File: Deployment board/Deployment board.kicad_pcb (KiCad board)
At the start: 2 copper layers, 43 x 51.5 mm, 28 parts, among them J1 Conn_01x04, J2 Conn_01x04, J3 Conn_01x02, J4 Conn_01x02, J5 Conn_01x02, J6 REMOVE BEFORE FLIGHT, M1 Motor_Servo, Q1 IRLR7843, Q2 IRLR7843, Q3 To be determined

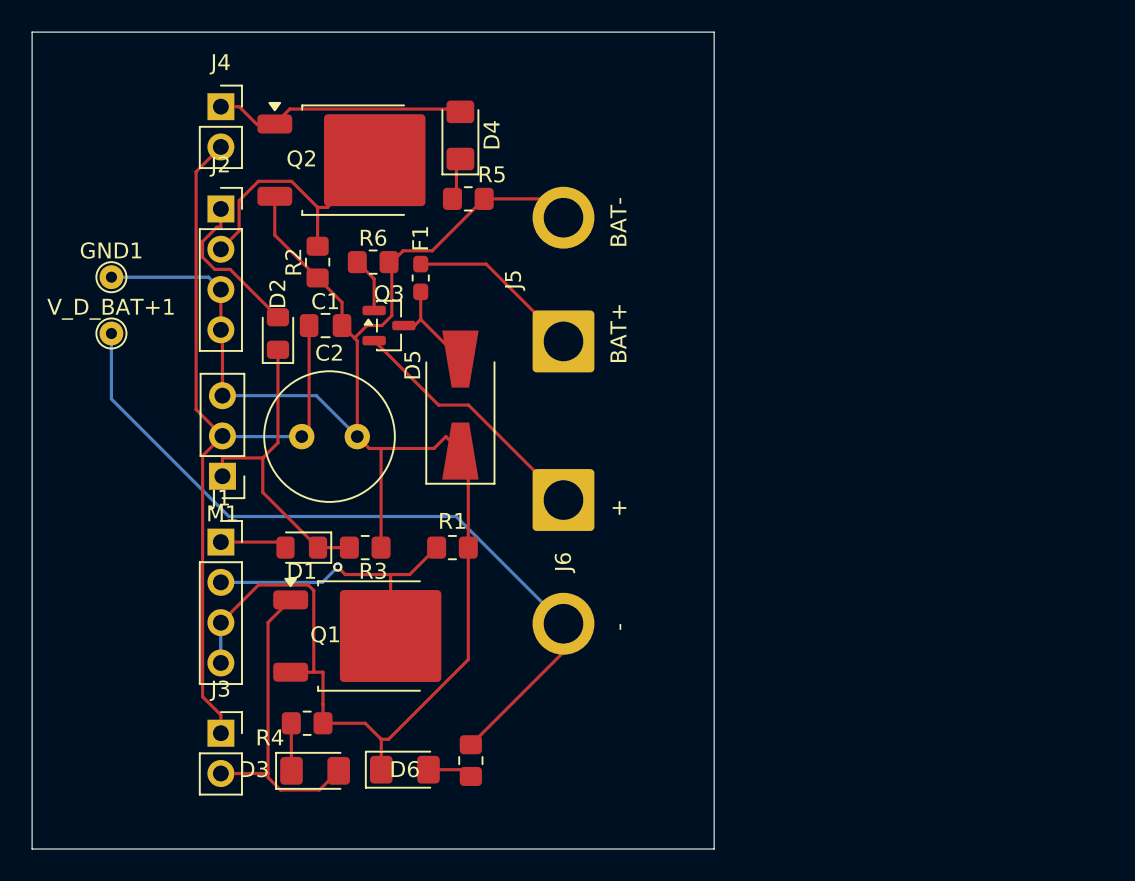
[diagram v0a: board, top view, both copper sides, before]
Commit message: jpush
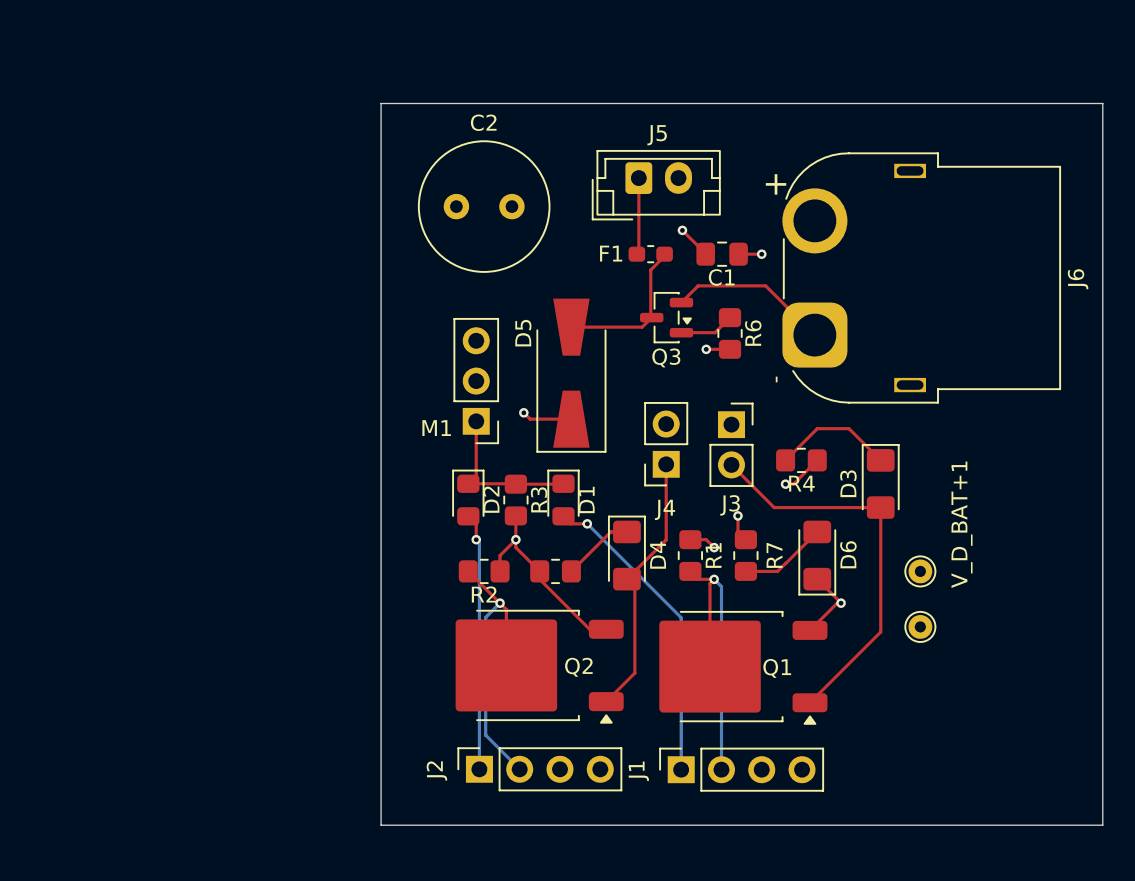
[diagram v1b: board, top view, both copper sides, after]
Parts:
- J5: footprint Connector_Wire:SolderWire-2sqmm_1x02_P7.8mm_D2mm_OD3.9mm -> Connector_JST:JST_EH_B2B-EH-A_1x02_P2.50mm_Vertical
- J6: footprint Connector_Wire:SolderWire-2sqmm_1x02_P7.8mm_D2mm_OD3.9mm -> Connector_AMASS:AMASS_XT60PW-F_1x02_P7.20mm_Horizontal
- moved GND1 55.6 mm to (71.5, 141.0), turned to 90 degrees
- moved V_D_BAT+1 53.2 mm to (71.5, 137.5)
- moved D3 40.0 mm to (69.0, 132.0), turned to -90 degrees
- moved J2 38.9 mm to (43.7, 150.0), turned to 90 degrees
- moved J3 37.6 mm to (59.6, 128.2)
- moved J4 36.0 mm to (55.5, 130.8), turned to 180 degrees
- moved R4 35.3 mm to (64.0, 130.5)
- moved Q2 33.6 mm to (46.7, 143.4), turned to 180 degrees
- moved J1 32.4 mm to (56.4, 150.0), turned to 90 degrees
- moved D6 29.3 mm to (65.0, 136.5), turned to 90 degrees
- moved D4 28.5 mm to (53.0, 136.5), turned to -90 degrees
- moved C1 25.4 mm to (59.0, 117.5), turned to 180 degrees
- moved R5 24.1 mm to (48.5, 137.5), turned to 180 degrees
- moved R6 22.9 mm to (59.5, 122.5), turned to -90 degrees
- moved Q1 22.7 mm to (59.5, 143.5), turned to 180 degrees
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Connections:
- C1 pad 1: V_Ｄ_BAT+ -> V_D_BAT+
- C2 pad 1: V_Ｄ_BAT+ -> V_D_BAT+
- J3 pad 1: V_Ｄ_BAT+ -> V_D_BAT+
- J4 pad 2: V_Ｄ_BAT+ -> V_D_BAT+
- M1 pad 2: V_Ｄ_BAT+ -> V_D_BAT+
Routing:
- net V_Ｄ_BAT+: track 51.5 -> 0.00 mm
- net V_D_BAT+: track 48.5 -> 70.4 mm, vias 0 -> 2
- net GND: track 120.9 -> 139.2 mm, vias 0 -> 7
- net Main_AV_PWM_Servo: track 4.22 -> 19.6 mm, vias 0 -> 1
- net Net-(D1-K): track 20.0 -> 10.2 mm
- net Backup_AV_PWM_Servo: track 9.99 -> 16.2 mm, vias 0 -> 1
- net Net-(J5-Pin_1): track 11.0 -> 4.85 mm
- net Net-(J6-A): track 16.1 -> 10.1 mm
- net Net-(D3-K): track 3.01 -> 7.66 mm
- net Net-(D3-A): track 20.0 -> 24.7 mm
- net Net-(D5-A2): track 6.50 -> 9.70 mm
- net Net-(D6-A): track 2.85 -> 5.53 mm
- net Backup_AV_FIRE: track 17.0 -> 18.7 mm, vias 0 -> 1
- net Net-(D4-K): track 3.07 -> 4.53 mm
- net Net-(D4-A): track 16.0 -> 16.9 mm
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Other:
- board size 43 x 51.5 mm -> 45.5 x 45.5 mm
- copper layers 2 -> 4
- board text removed: "+"
- board text removed: "-"
- board text removed: "BAT+"
- board text removed: "BAT-"

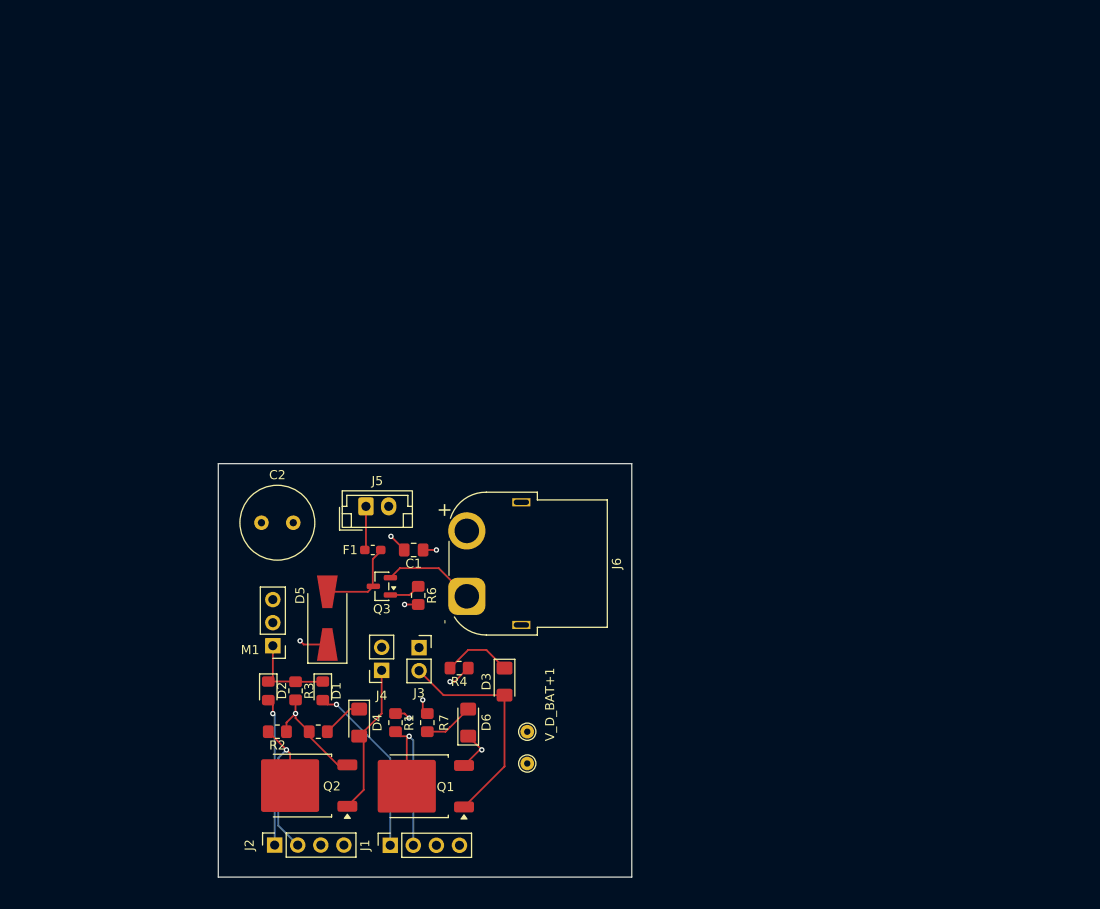
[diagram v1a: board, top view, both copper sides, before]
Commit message: finish deployment pcb
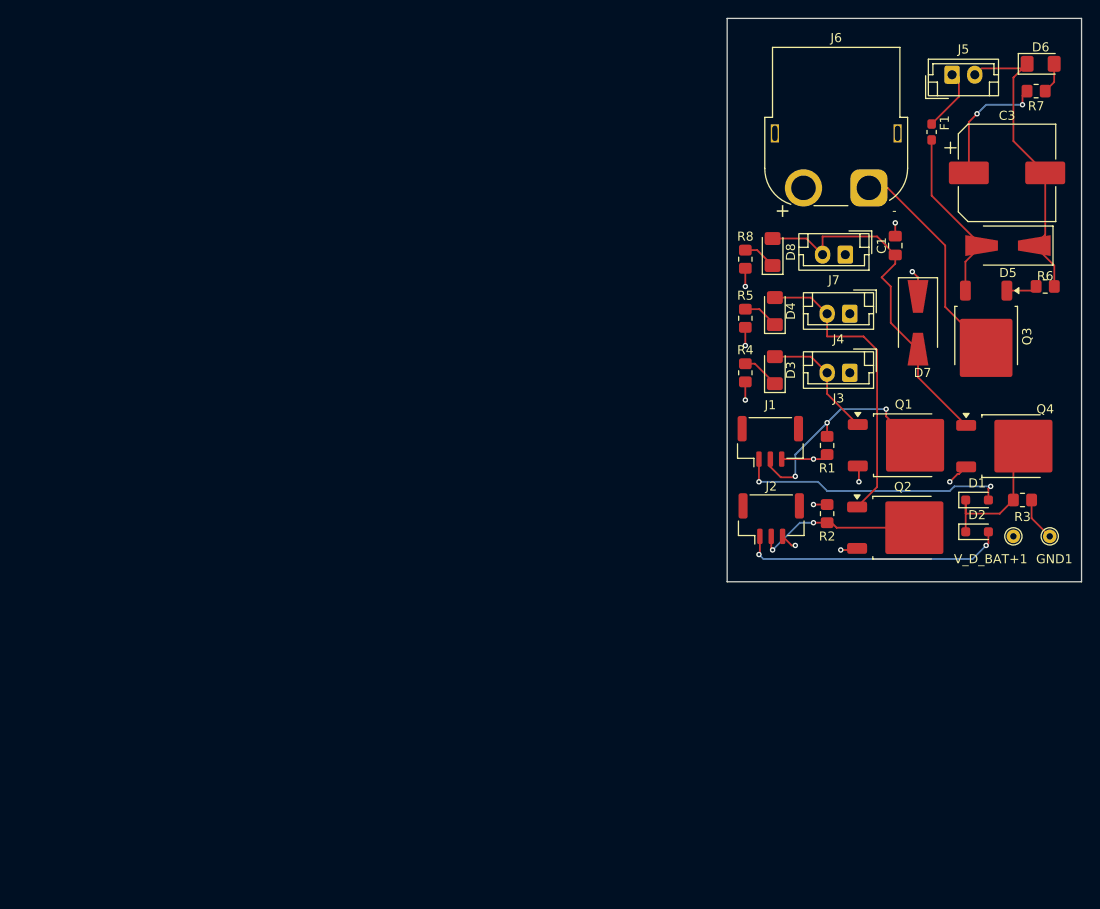
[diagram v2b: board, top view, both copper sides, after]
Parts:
- removed C2: 1000u, Capacitor_THT:C_Radial_D8.0mm_H7.0mm_P3.50mm
- removed M1: Motor_Servo, Connector_PinHeader_2.54mm:PinHeader_1x03_P2.54mm_Vertical
- added C3: 667-EEH-ZS1E102UP(1000u), Capacitor_SMD:CP_Elec_10x14.3, F.Cu at (124.3, 76.0)
- added D7: SS54, Diode_SMD:D_SMA-SMB_Universal_Handsoldering, F.Cu at (114.5, 92.5)
- added D8: LED, LED_SMD:LED_1206_3216Metric_Pad1.42x1.75mm_HandSolder, F.Cu at (98.5, 84.7)
- added J7: Conn_01x02, Connector_JST:JST_EH_B2B-EH-A_1x02_P2.50mm_Vertical, F.Cu at (106.5, 85.0)
- added Q4: IRLR7843, Package_TO_SOT_SMD:TO-252-2, F.Cu at (124.8, 106.1)
- added R8: 3.3k, Resistor_SMD:R_0805_2012Metric_Pad1.20x1.40mm_HandSolder, F.Cu at (95.5, 85.5)
- D1, D2: value D_Schottky -> 78-SD101CWS-HE3_A-08; footprint Diode_SMD:D_0805_2012Metric_Pad1.15x1.40mm_HandSolder -> Diode_SMD:D_SOD-323_HandSoldering
- D6: value B_3V3 -> LED
- J1, J2: footprint Connector_PinSocket_2.54mm:PinSocket_1x04_P2.54mm_Vertical -> Connector_JST:JST_GH_BM03B-GHS-TBT_1x03-1MP_P1.25mm_Vertical
- J3, J4: footprint Connector_PinSocket_2.54mm:PinSocket_1x02_P2.54mm_Vertical -> Connector_JST:JST_EH_B2B-EH-A_1x02_P2.50mm_Vertical
- Q3: value To be determined -> RM40P40LD; footprint Package_TO_SOT_SMD:SOT-23 -> Package_TO_SOT_SMD:TO-252-2
- R7: value 1k -> 3.3k
- moved R7 96.5 mm to (127.5, 67.0), turned to 180 degrees
- moved D6 96.0 mm to (128.0, 64.0), turned to 0 degrees
- moved D5 85.4 mm to (124.4, 84.0), turned to 180 degrees
- moved R3 82.7 mm to (126.0, 112.0), turned to 0 degrees
- moved J5 80.1 mm to (118.2, 65.2)
- moved D2 79.9 mm to (121.0, 115.5), turned to 0 degrees
- moved R6 76.9 mm to (128.5, 88.5), turned to 0 degrees
- moved F1 76.8 mm to (116.0, 71.5), turned to -90 degrees
- moved D1 75.0 mm to (121.0, 112.0), turned to 0 degrees
- moved Q2 72.0 mm to (112.8, 115.0), turned to 0 degrees
- moved Q3 72.0 mm to (122.0, 94.0), turned to -90 degrees
- moved R5 65.4 mm to (95.5, 92.0), turned to -90 degrees
- moved J2 65.4 mm to (98.3, 114.0), turned to 0 degrees
- moved Q1 65.3 mm to (112.9, 106.0), turned to 0 degrees
- moved R2 65.1 mm to (104.5, 113.5), turned to 90 degrees
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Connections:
- C1 pad 1: V_D_BAT+ -> Net-(D7-A)
- C1 pad 2: GND -> V_D_BAT+
- J4 pad 1: Net-(D4-A) -> V_D_BAT+
- J4 pad 2: V_D_BAT+ -> Net-(D4-A)
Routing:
- net GND: track 139.2 -> 57.6 mm, vias 7 -> 9
- net V_D_BAT+: track 70.4 -> 18.4 mm, vias 2 -> 4
- net Net-(D7-A): track 0.00 -> 40.3 mm
- net Net-(D4-A): track 16.9 -> 33.3 mm
- net Net-(J6-A): track 10.1 -> 24.2 mm
- net Backup_AV_PWM_Servo: track 16.2 -> 29.5 mm, vias 1 -> 2
- net Net-(D3-A): track 24.7 -> 13.6 mm
- net Main_AV_PWM_Servo: track 19.6 -> 30.2 mm, vias 1 -> 2
- net Net-(D5-A2): track 9.70 -> 19.6 mm
- net Main_AV_FIRE: track 19.5 -> 25.4 mm, vias 1 -> 3
- net Net-(D1-K): track 10.2 -> 15.7 mm
- net Net-(D8-K): track 0.00 -> 3.70 mm
- net Net-(D3-K): track 7.66 -> 4.16 mm
- net Net-(D6-A): track 5.53 -> 3.41 mm
- net Net-(J5-Pin_1): track 4.85 -> 6.37 mm
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- added copper zone on In2.Cu, net GND
- added copper zone on In1.Cu, net V_D_BAT+
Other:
- board size 45.5 x 45.5 mm -> 39 x 62 mm
